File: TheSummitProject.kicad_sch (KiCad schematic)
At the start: 37 parts, among them IC1 STM32U5F7VJT6, J1 Cortex SWD, SW1 SW_SPDT, U10 TS3USB30EDGSR, U2 USBLC6-2SC6, U3 USBLC6-2SC6, Y1 16Mhz, Y2 32.768Khz

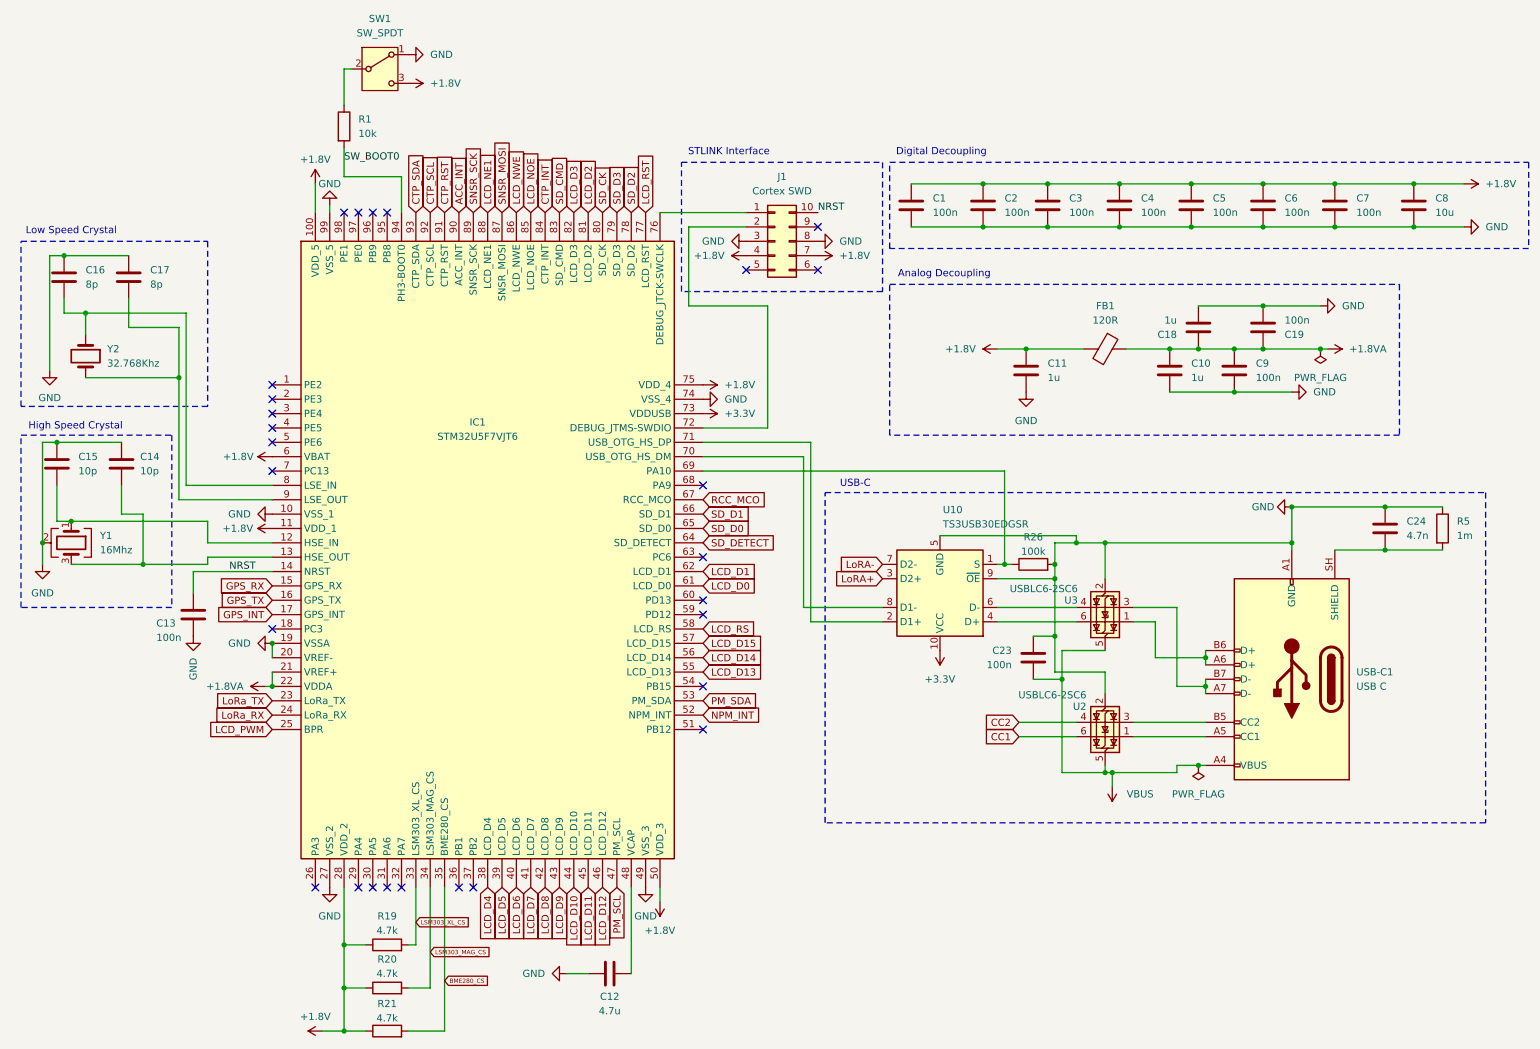
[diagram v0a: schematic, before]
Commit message: pcb draft, cleaned up schematic
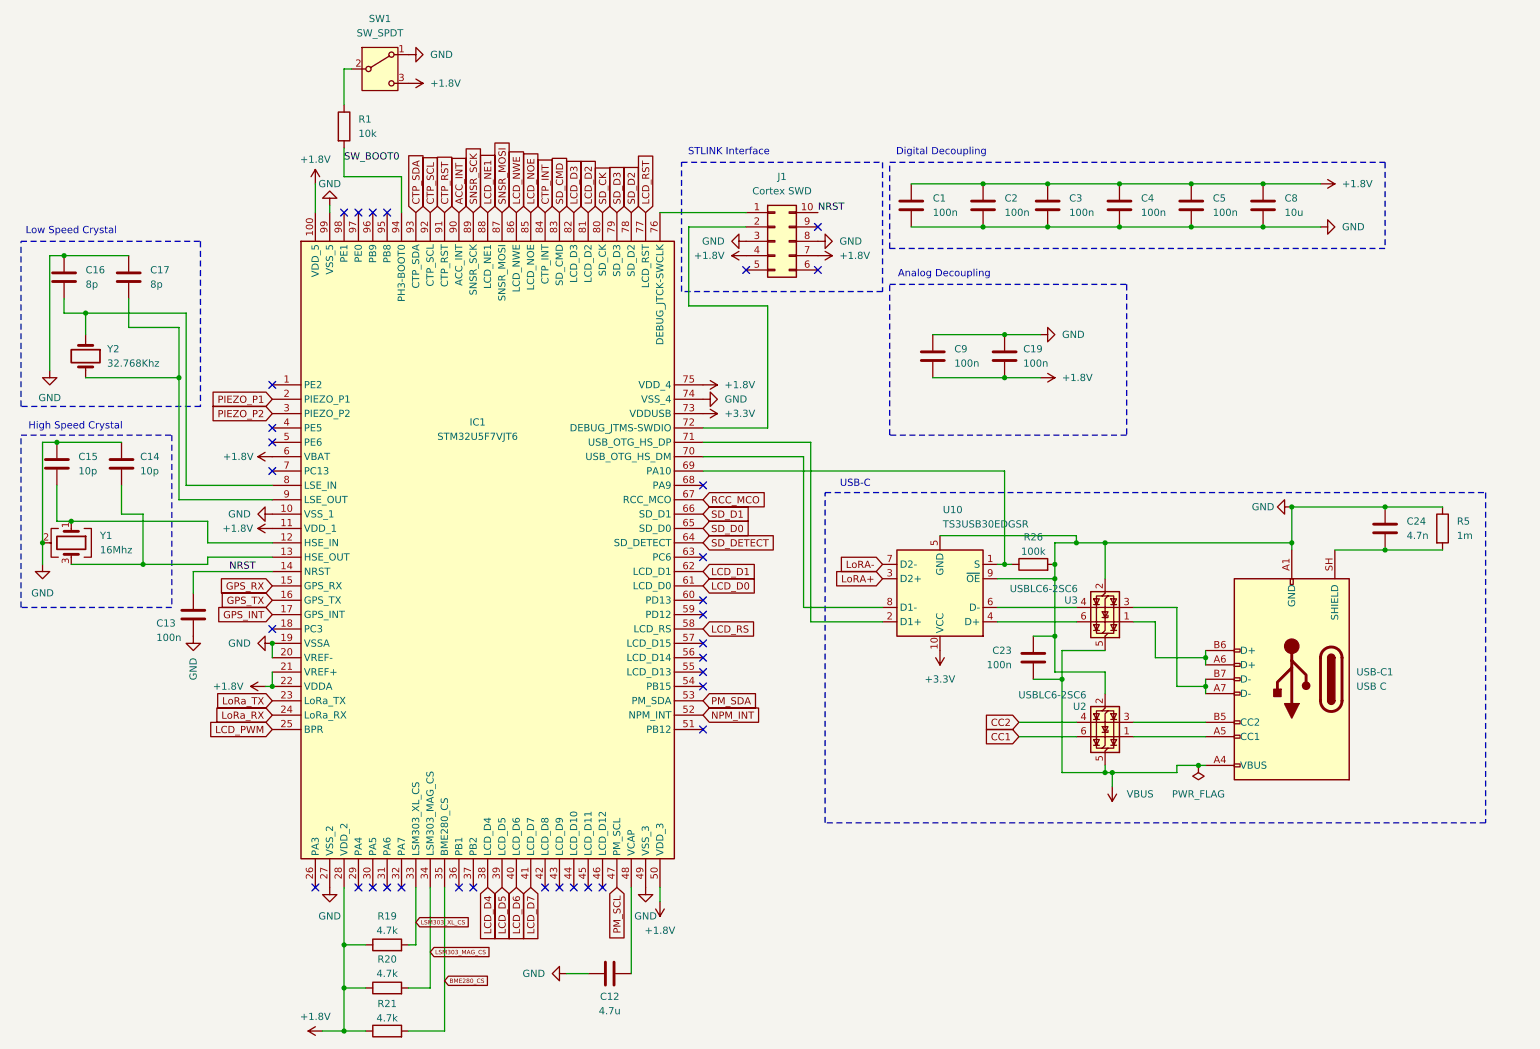
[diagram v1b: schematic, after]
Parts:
- removed C10, C11, C18: 1u, Capacitor_SMD:C_0603_1608Metric, symbol Device:C
- removed C6, C7: 100n, Capacitor_SMD:C_0603_1608Metric, symbol Device:C
- removed FB1: 120R, Inductor_SMD:L_0603_1608Metric, symbol Device:FerriteBead
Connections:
- net +1.8V: now also C19.1, C9.2, IC1.21 (VREF+), IC1.22 (VDDA)
- net GND: now also C9.1; no longer C9.2
- net PIEZO_P1: now reaches IC1.2 (PIEZO_P1)
- net PIEZO_P2: now reaches IC1.3 (PIEZO_P2)
- removed net +1.8VA: C19.1, C9.1, IC1.21 (VREF+), IC1.22 (VDDA)
- net LCD_D10: no longer names the net of IC1.44 (LCD_D10)
- net LCD_D11: no longer names the net of IC1.45 (LCD_D11)
- net LCD_D12: no longer names the net of IC1.46 (LCD_D12)
- net LCD_D13: no longer names the net of IC1.55 (LCD_D13)
- net LCD_D14: no longer names the net of IC1.56 (LCD_D14)
- net LCD_D15: no longer names the net of IC1.57 (LCD_D15)
- net LCD_D8: no longer names the net of IC1.42 (LCD_D8)
- net LCD_D9: no longer names the net of IC1.43 (LCD_D9)
- no-connect marks 27 -> 33
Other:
- moved on the sheet: C8
